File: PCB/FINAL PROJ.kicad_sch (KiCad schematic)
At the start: 23 parts, among them J1 left side, J10 PIR_SENSOR, J11 BUTTON, J12 RGB_LED, J13 HX711, J14 BUZZER, J15 LCD display/OLED, J2 right side, J3 5V, J4 3.3V, J6 SERVO, J7 ULTRASONIC_1, J8 RTC_MODULE, J9 ULTRASONIC_2, Q1 IRLZ44N

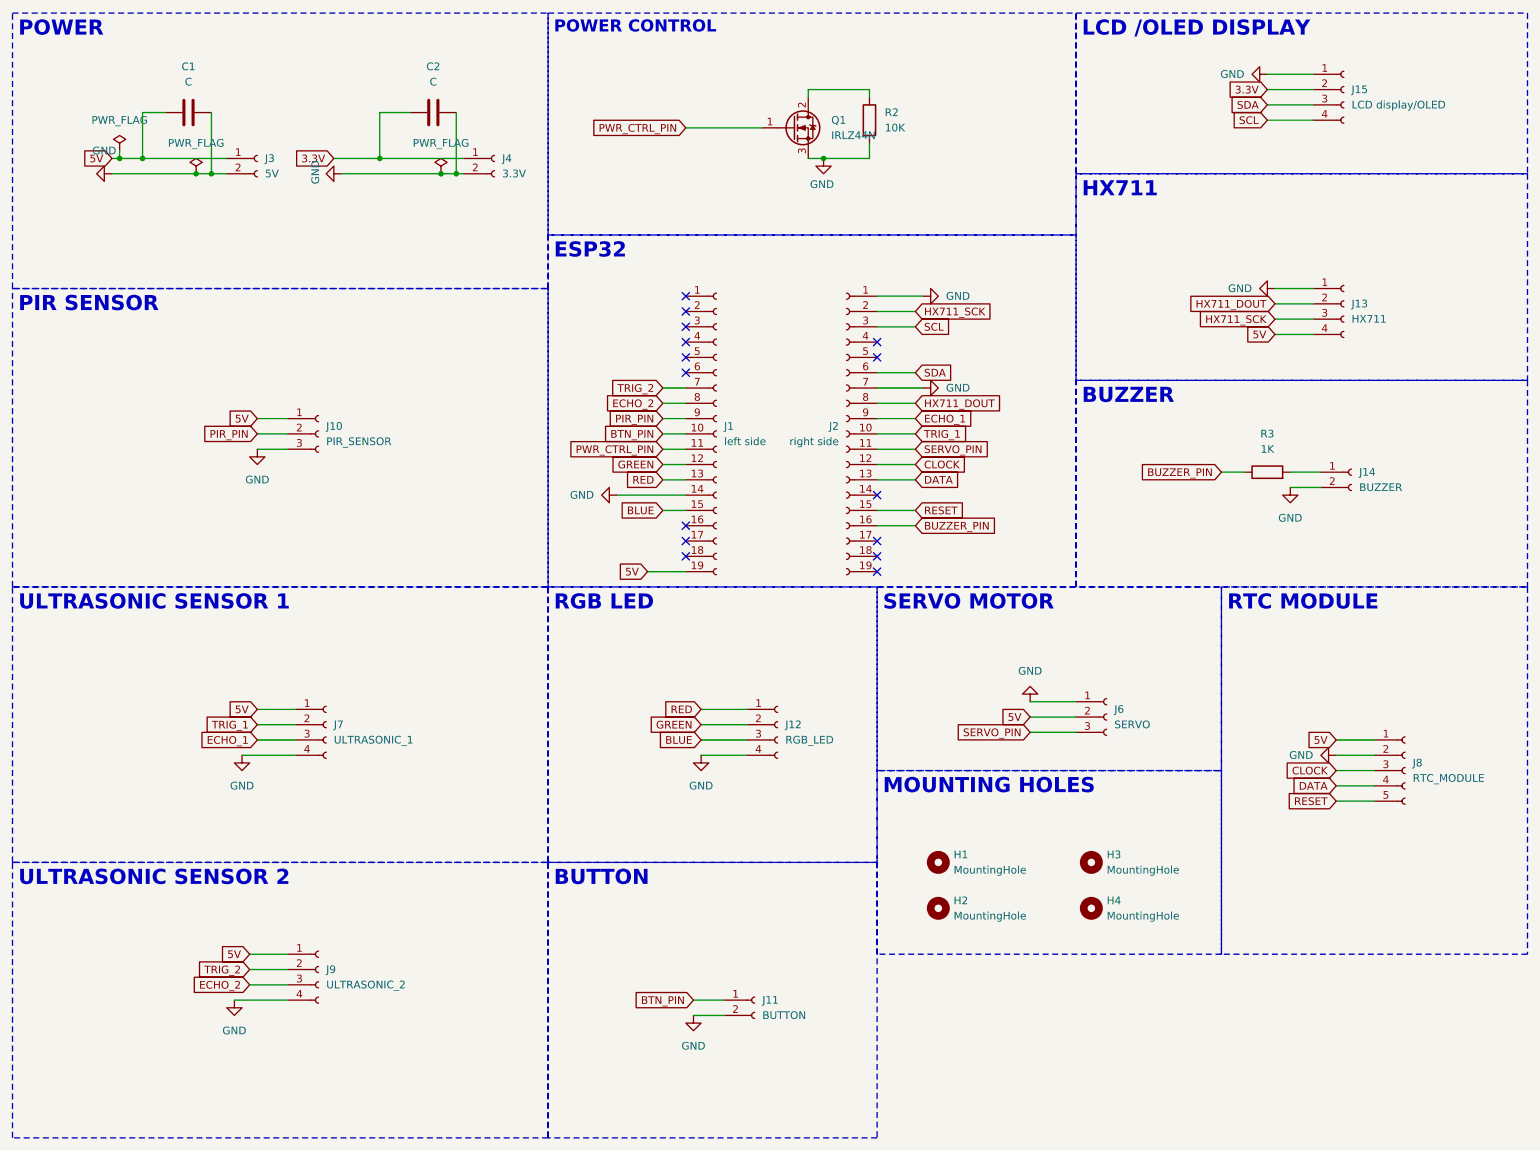
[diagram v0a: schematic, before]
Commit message: refactor: updated pcb
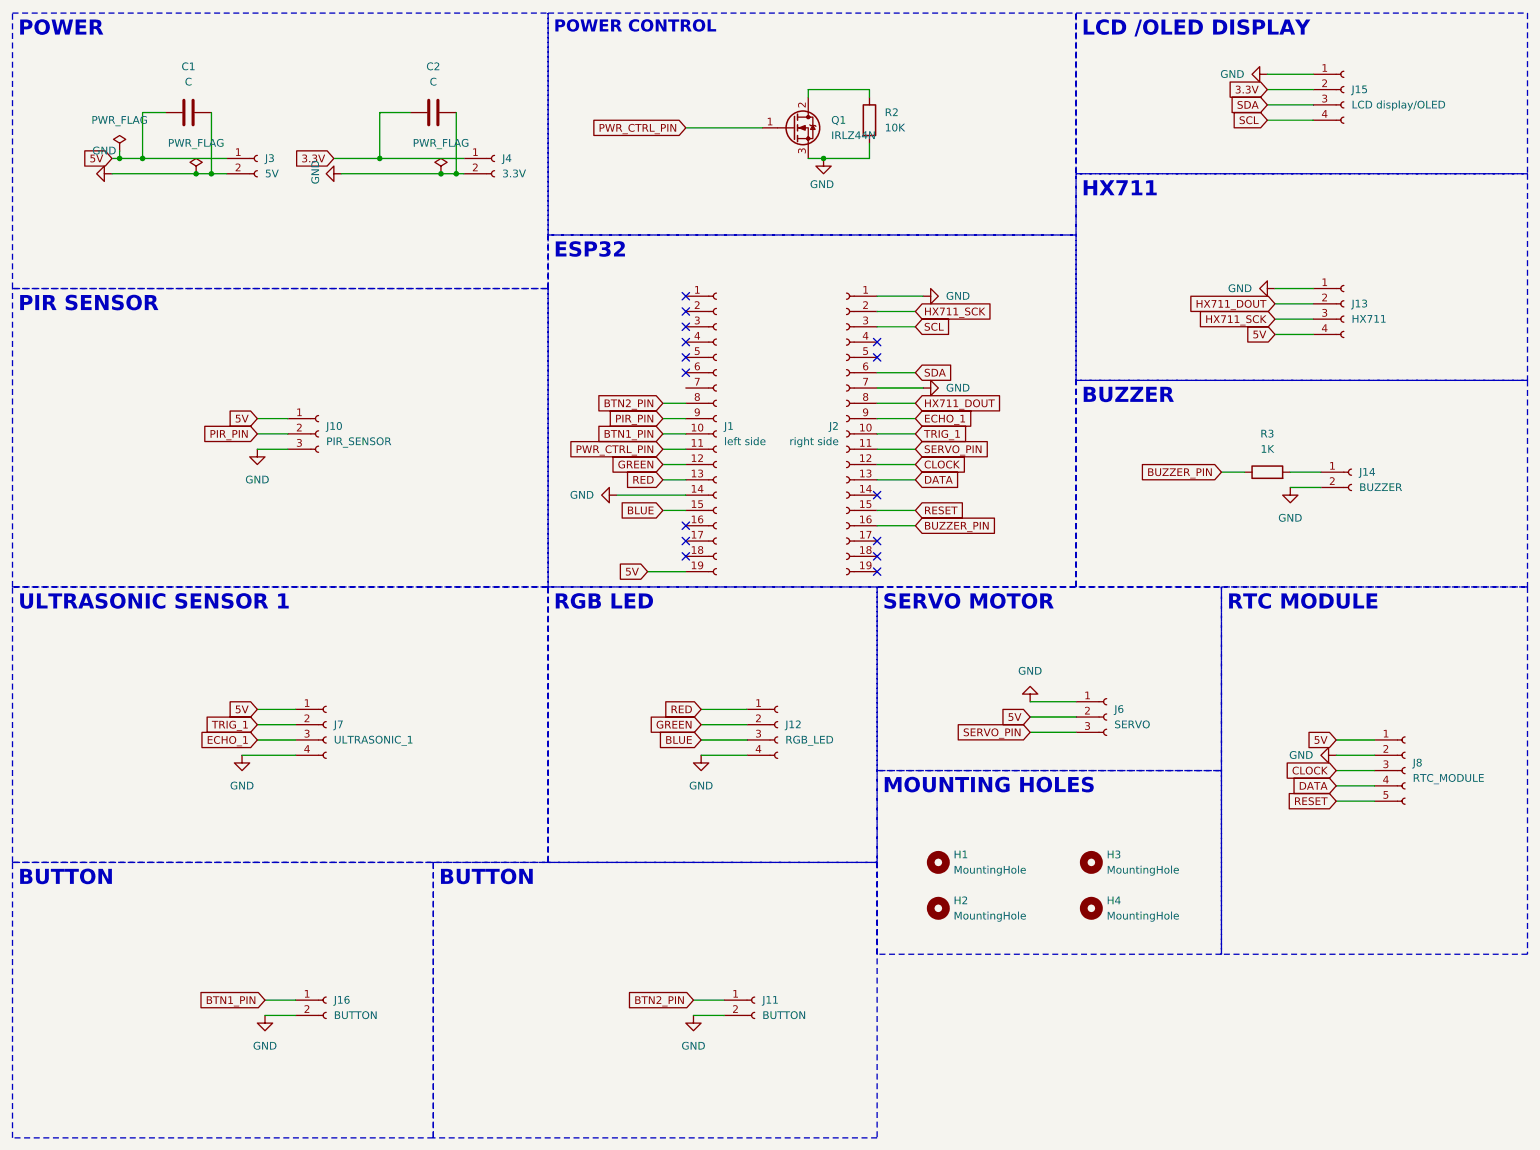
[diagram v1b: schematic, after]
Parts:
- removed J9: ULTRASONIC_2, Connector_JST:JST_EH_B4B-EH-A_1x04_P2.50mm_Vertical, symbol Connector:Conn_01x04_Socket
- added J16: BUTTON, Connector_JST:JST_EH_B2B-EH-A_1x02_P2.50mm_Vertical, symbol Connector:Conn_01x02_Socket
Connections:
- net GND: now also J16.2 (Pin_2)
- net BTN_PIN renamed BTN1_PIN
- net BTN1_PIN: now also J16.1 (Pin_1); no longer J11.1 (Pin_1)
- net ECHO_2 renamed BTN2_PIN
- net BTN2_PIN: now also J11.1 (Pin_1)
- net TRIG_2: no longer names the net of J1.7 (Pin_7)
